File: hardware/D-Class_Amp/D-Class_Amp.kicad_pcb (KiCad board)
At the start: 2 copper layers, 180 x 65 mm, 98 parts, among them J101 P_IN, J102 AudioJack2, M3 MountingHole_Pad, Q501 PHP23NQ11T, Q502 PHP23NQ11T, Q503 PHP23NQ11T, Q504 PHP23NQ11T, U101 NCP1117-12_TO252, U102 MCP1799T-5002H_TT, U201 LM324, U301 TL972, U302 LMV393, U501 IR21834, U502 IR21834

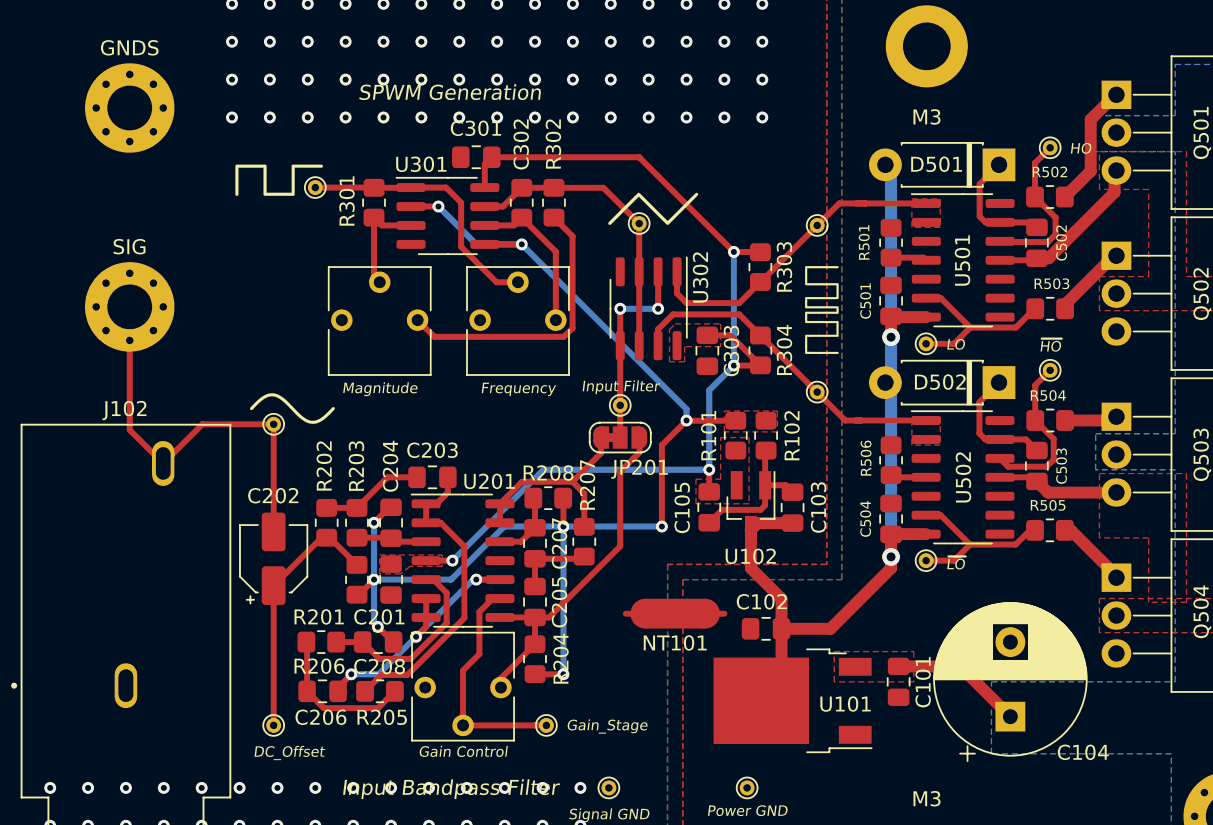
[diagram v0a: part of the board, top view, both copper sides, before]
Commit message: goddam GNDS bck_plane
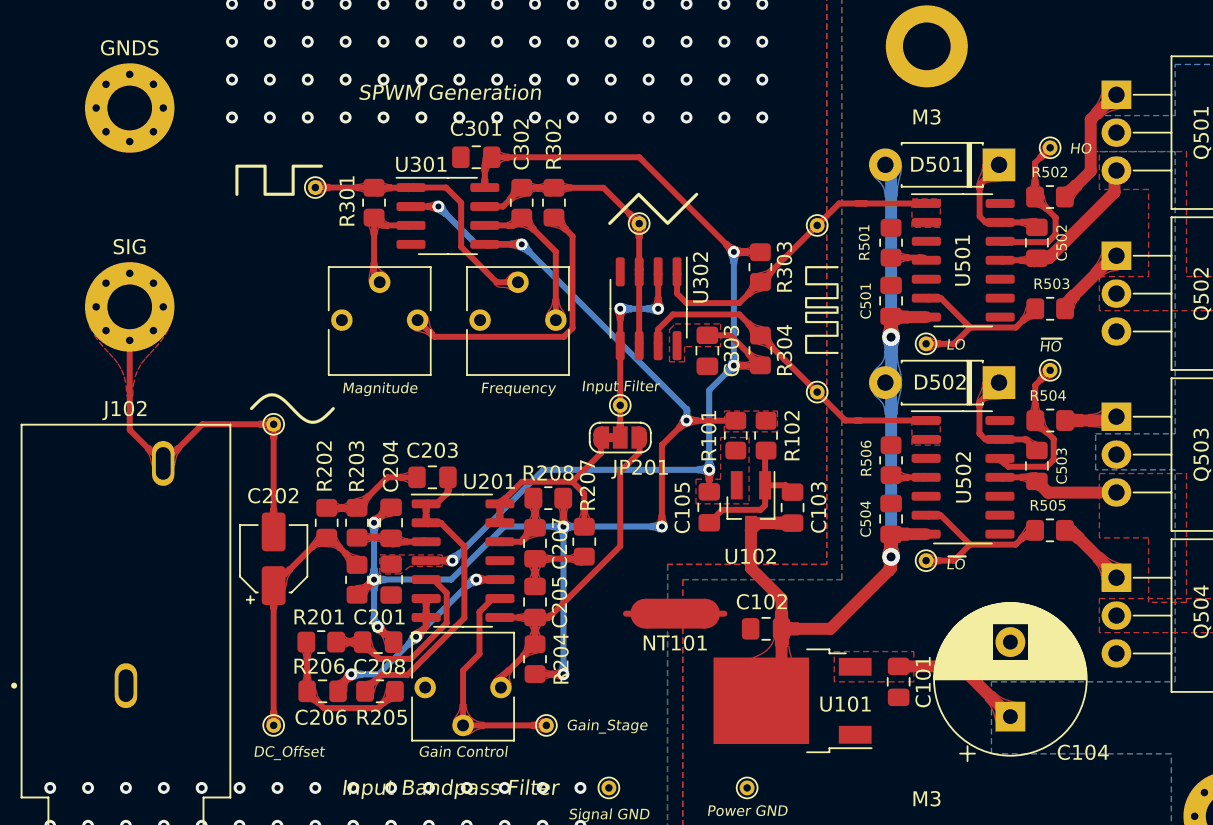
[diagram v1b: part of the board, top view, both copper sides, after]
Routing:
- net GNDS: vias 60 -> 120
- net (no net): vias 60 -> 0
- added copper zone on B.Cu, net GNDS
- removed copper zone on B.Cu, net (none)
